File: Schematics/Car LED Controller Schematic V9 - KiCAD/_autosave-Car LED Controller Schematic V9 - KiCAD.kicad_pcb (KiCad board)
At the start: 2 copper layers, 101.9 x 70 mm, 25 parts, among them J1 5V Power In, J2 Select Button, J3 LCD, Relay, LED Signal, J4 ZSS-108-01-F-D-506, J5 DRL, Horn Sense, J6 Reset Button, U1 ESP32-DEVKITC-32D, U2 BOB-12009, U3 PC817X3NSZ9F, U4 PC817X3NSZ9F, U5 PC817X3NSZ9F

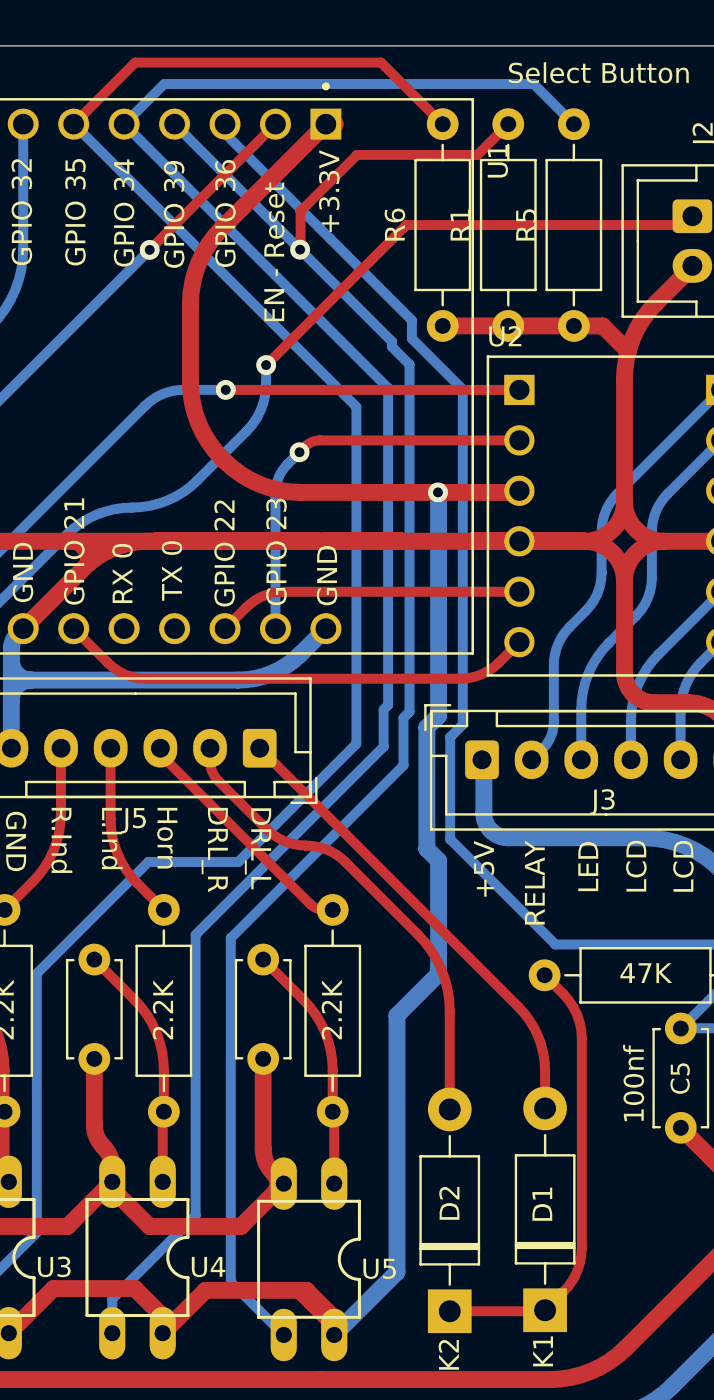
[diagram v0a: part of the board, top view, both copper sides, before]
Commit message: PCB and Schematic updates
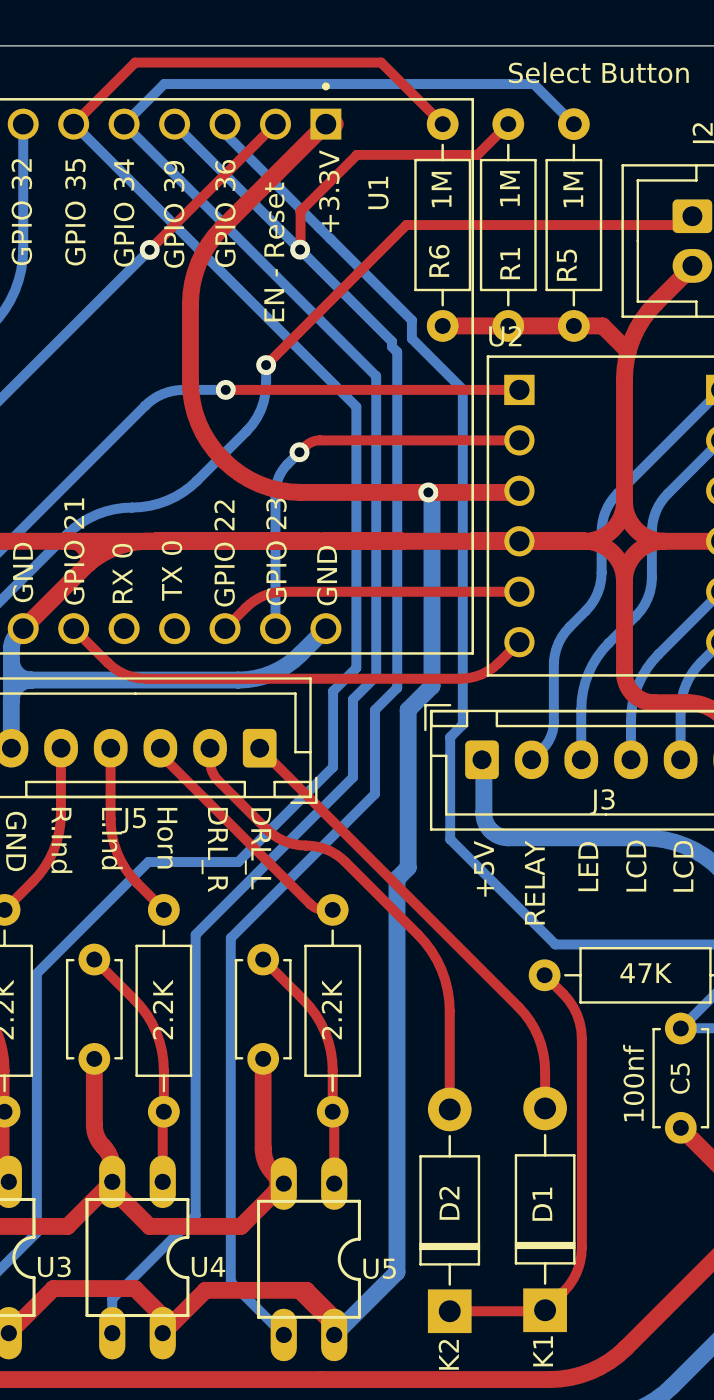
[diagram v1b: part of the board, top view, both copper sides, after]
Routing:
- net +3.3V: track 108.1 -> 107.5 mm
- net /Horn: track 85.5 -> 85.0 mm
